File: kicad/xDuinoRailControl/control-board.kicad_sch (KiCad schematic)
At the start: 3 parts, among them J3 OLED_SOCKET, SW1 SW_Nidec_CAS-120A1, U2 XIAO-ESP32C3

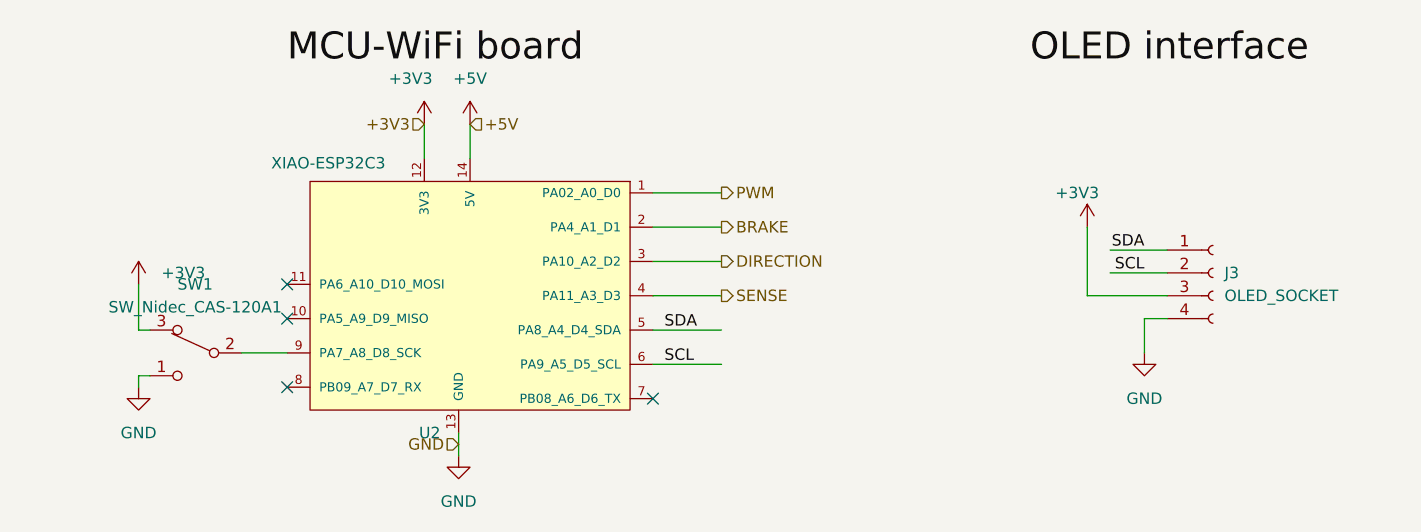
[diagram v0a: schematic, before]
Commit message: Add encoder
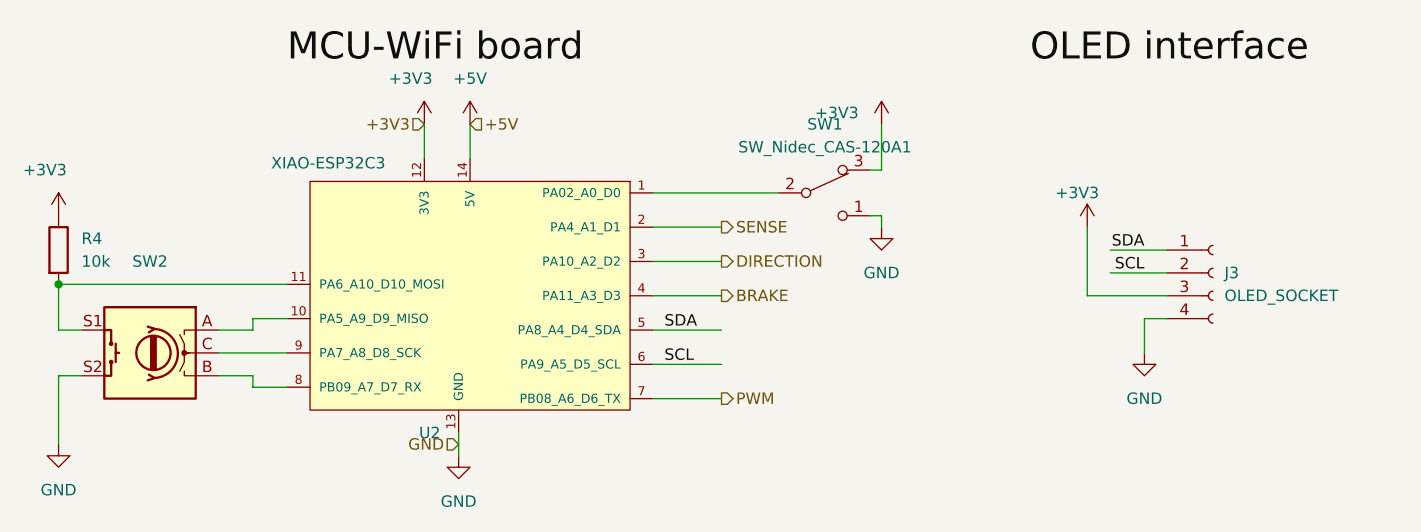
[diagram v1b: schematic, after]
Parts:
- added R4: 10k, symbol Device:R
- added SW2: RotaryEncoder_Switch, Rotary_Encoder:RotaryEncoder_Alps_EC11E-Switch_Vertical_H20mm_CircularMountingHoles, symbol Device:RotaryEncoder_Switch
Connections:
- net +3V3: now also R4.1
- net BRAKE: now also U2.4 (PA11_A3_D3); no longer U2.2 (PA4_A1_D1)
- net GND: now also SW2.S2
- net PWM: now also U2.7 (PB08_A6_D6_TX); no longer U2.1 (PA02_A0_D0)
- net SENSE: now also U2.2 (PA4_A1_D1); no longer U2.4 (PA11_A3_D3)
- net at U2.9 (PA7_A8_D8_SCK): now also SW2.C; no longer SW1.2 (B)
- net at U2.10 (PA5_A9_D9_MISO): now also SW2.A
- net at U2.11 (PA6_A10_D10_MOSI): now also R4.2, SW2.S1
- net at U2.8 (PB09_A7_D7_RX): now also SW2.B
- new net: SW1.2 (B), U2.1 (PA02_A0_D0)
- no-connect marks 4 -> 0
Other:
- moved on the sheet: SW1
